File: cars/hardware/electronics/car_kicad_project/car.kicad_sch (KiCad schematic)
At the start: 10 parts, among them M1 Motor_DC, M2 Motor_DC, M3 Motor_DC, M4 Motor_DC, U1 MOUDLE-SEEEDUINO-XIAO-ESP32S3, U2 Adafruit motor driver DRV8833, U3 Purecrea MPU-6050

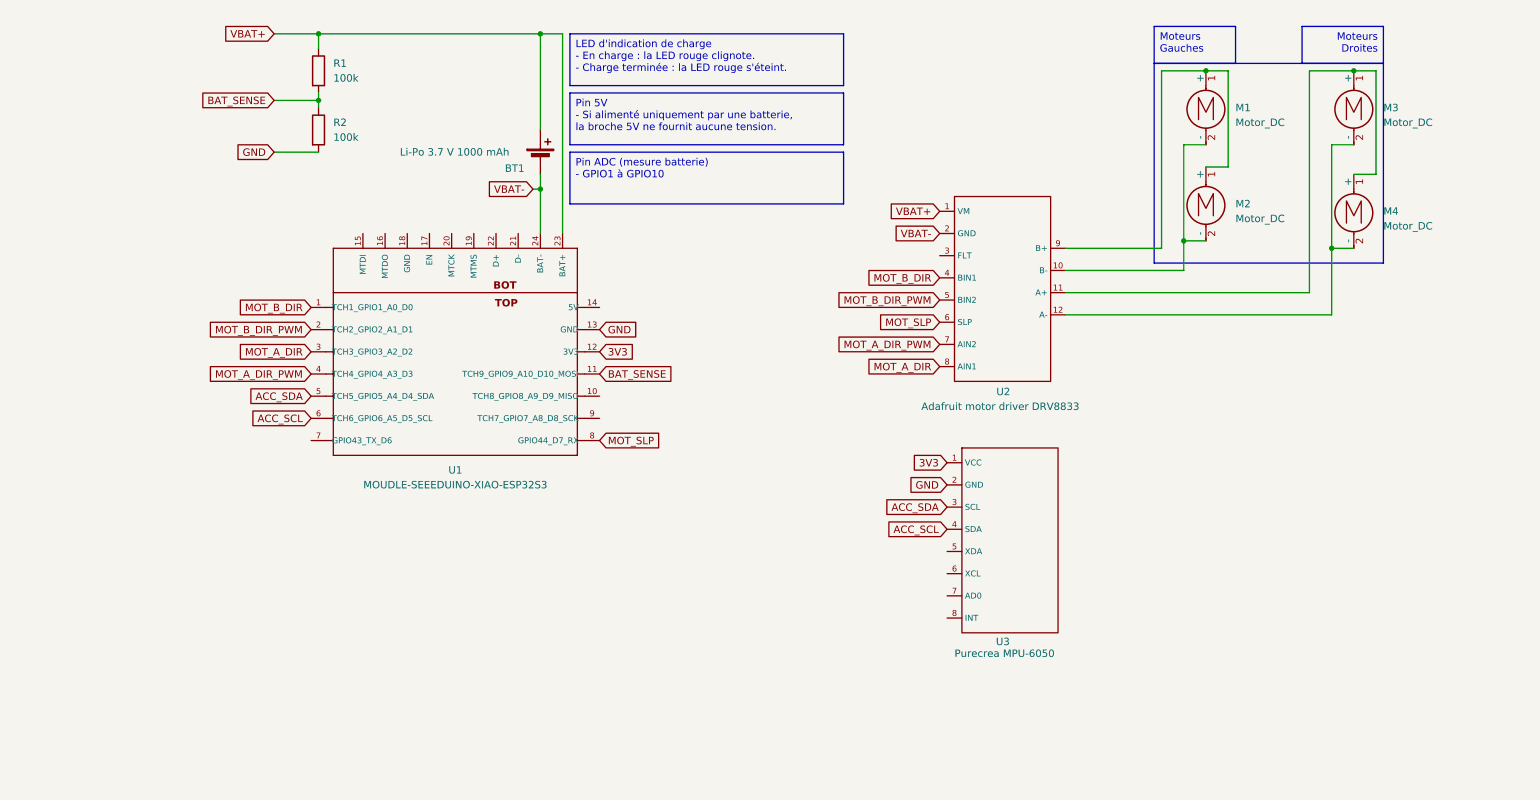
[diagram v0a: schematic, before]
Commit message: placement + route ok
miss the outline
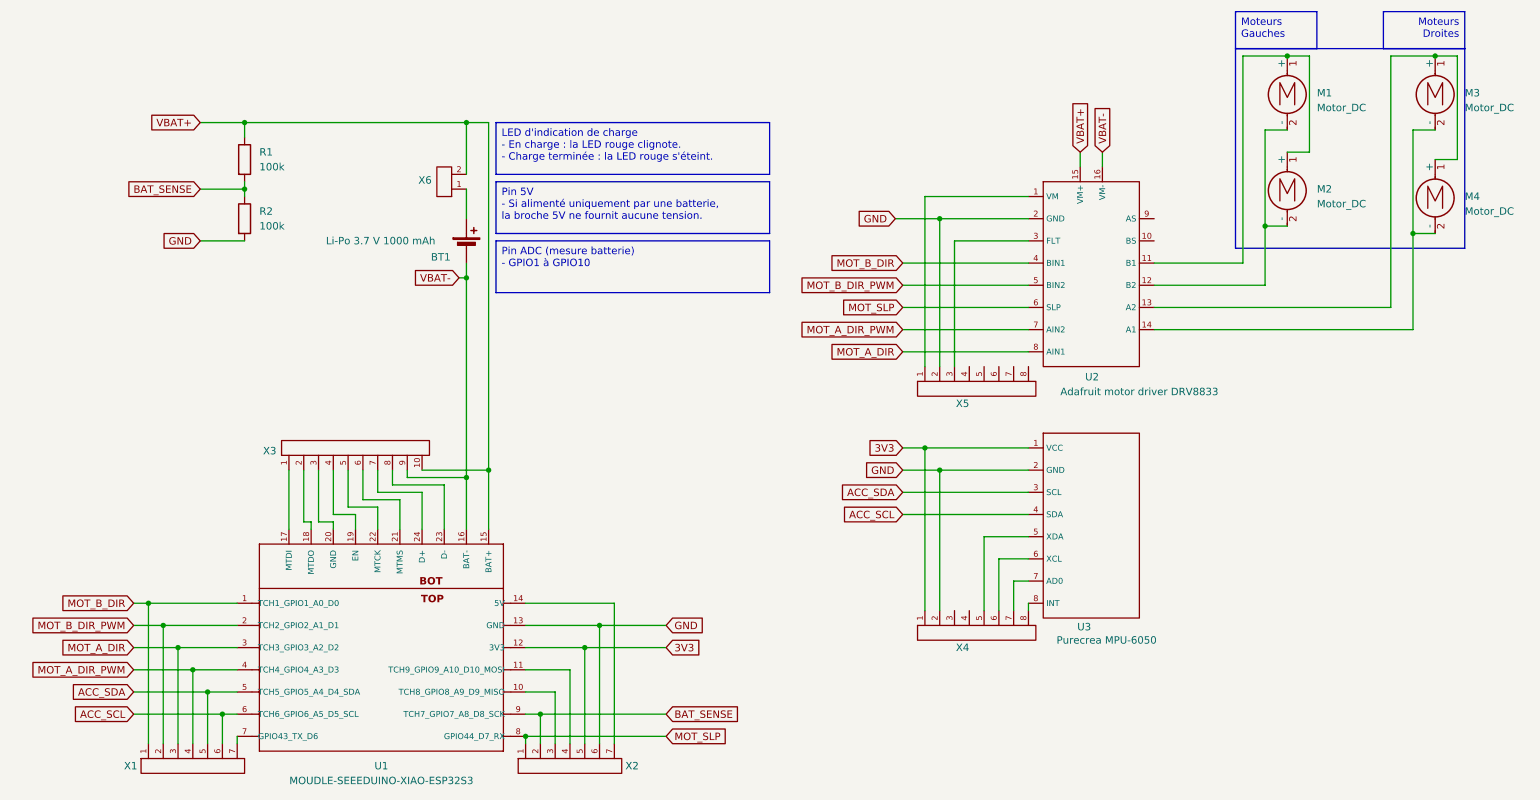
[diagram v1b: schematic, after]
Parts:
- added X1, X2: ~, pin_header:PinHeader_1x07_P2.54mm_Vertical, symbol adafruit_perso:pin_header_7
- added X3: ~, pin_header:PinHeader_1x10_P2.54mm_Vertical, symbol adafruit_perso:pin_header_10
- added X4, X5: ~, pin_header:PinHeader_1x08_P2.54mm_Vertical, symbol adafruit_perso:pin_header_8
- added X6: ~, pin_header:PinHeader_1x02_P2.54mm_Vertical, symbol adafruit_perso:pin_header_2
- BT1, M1, M2, M3, M4: footprint (none) -> Connector_JST:JST_PH_B2B-PH-K_1x02_P2.00mm_Vertical
- R1, R2: footprint (none) -> Resistor_THT:R_Axial_DIN0309_L9.0mm_D3.2mm_P15.24mm_Horizontal
- U1: footprint MOUDLE14P-SMD-2.54-21X17.8MM -> xiao_esp32s3:XIAO-ESP32S3-SMD
- U2: footprint (none) -> adafruit_drv8833:adafruit_drv8833
- U3: footprint (none) -> adafruit_drv8833:pucrea_mpu_6050
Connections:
- net 3V3: now also X2.5, X4.1
- net ACC_SCL: now also X1.6
- net ACC_SDA: now also X1.5
- net BAT_SENSE: now also U1.9 (TCH7_GPIO7_A8_D8_SCK), X2.2; no longer U1.11 (TCH9_GPIO9_A10_D10_MOSI)
- net GND: now also U2.2 (GND), X2.6, X4.2, X5.2
- net MOT_A_DIR: now also X1.3
- net MOT_A_DIR_PWM: now also X1.4
- net MOT_B_DIR: now also X1.1
- net MOT_B_DIR_PWM: now also X1.2
- net MOT_SLP: now also X2.1
- net VBAT+: now also U1.15 (BAT+), U2.15 (VM+), X3.10, X6.2; no longer BT1.1 (+), U1.23 (BAT+), U2.1 (VM)
- net VBAT-: now also U1.16 (BAT-), U2.16 (VM-), X3.9; no longer U1.24 (BAT-), U2.2 (GND)
- net at U3.5 (XDA): now also X4.5
- net at U3.6 (XCL): now also X4.6
- net at U3.7 (AD0): now also X4.7
- net at U3.8 (INT): now also X4.8
- net at M3.1 (+), M4.1 (+): now also U2.13 (A2); no longer U2.11 (A+)
- net at M3.2 (-), M4.2 (-): now also U2.14 (A1); no longer U2.12 (A-)
- net at M1.1 (+), M2.1 (+): now also U2.11 (B1); no longer U2.9 (B+)
- net at M1.2 (-), M2.2 (-): now also U2.12 (B2); no longer U2.10 (B-)
- net at U1.10 (TCH8_GPIO8_A9_D9_MISO): now also X2.3
- net at U1.14 (5V): now also X2.7
- net at U1.17 (MTDI): now also X3.1
- net at U1.18 (MTDO): now also X3.2
- net at U1.19 (EN): now also X3.4
- net at U1.20 (GND): now also X3.3
- net at U1.21 (MTMS): now also X3.6
- net at U1.22 (MTCK): now also X3.5
- net at U1.7 (GPIO43_TX_D6): now also X1.7
- net at U2.3 (FLT): now also X5.3
- new net: BT1.1 (+), X6.1
- new net: U1.11 (TCH9_GPIO9_A10_D10_MOSI), X2.4
- new net: U1.23 (D-), X3.8
- new net: U1.24 (D+), X3.7
- new net: U2.1 (VM), X5.1
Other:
- moved on the sheet: BT1, M1, M2, M3, M4, R1, R2, U1, U3

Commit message: finish esp32 module pcb
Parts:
- U1: footprint xiao_esp32s3:XIAO-ESP32S3-SMD -> MOUDLE14P-SMD-2.54-21X17.8MM
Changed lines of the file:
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@@
 			)
 		)
-		(property "Footprint" "xiao_esp32s3:XIAO-ESP32S3-SMD"
+		(property "Footprint" "MOUDLE14P-SMD-2.54-21X17.8MM"
 			(at 85.09 142.24 0)
 			(effects
